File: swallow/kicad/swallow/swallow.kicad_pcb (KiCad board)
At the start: 2 copper layers, 35 parts, among them J1 Raspberry_Pi_2_3, J10 evens, J2 echo2, J3 ground, J4 VCC, J5 echo3, J6 echo4, J7 echo1, J8 power terminal, J9 odds, SW1 SW_Push

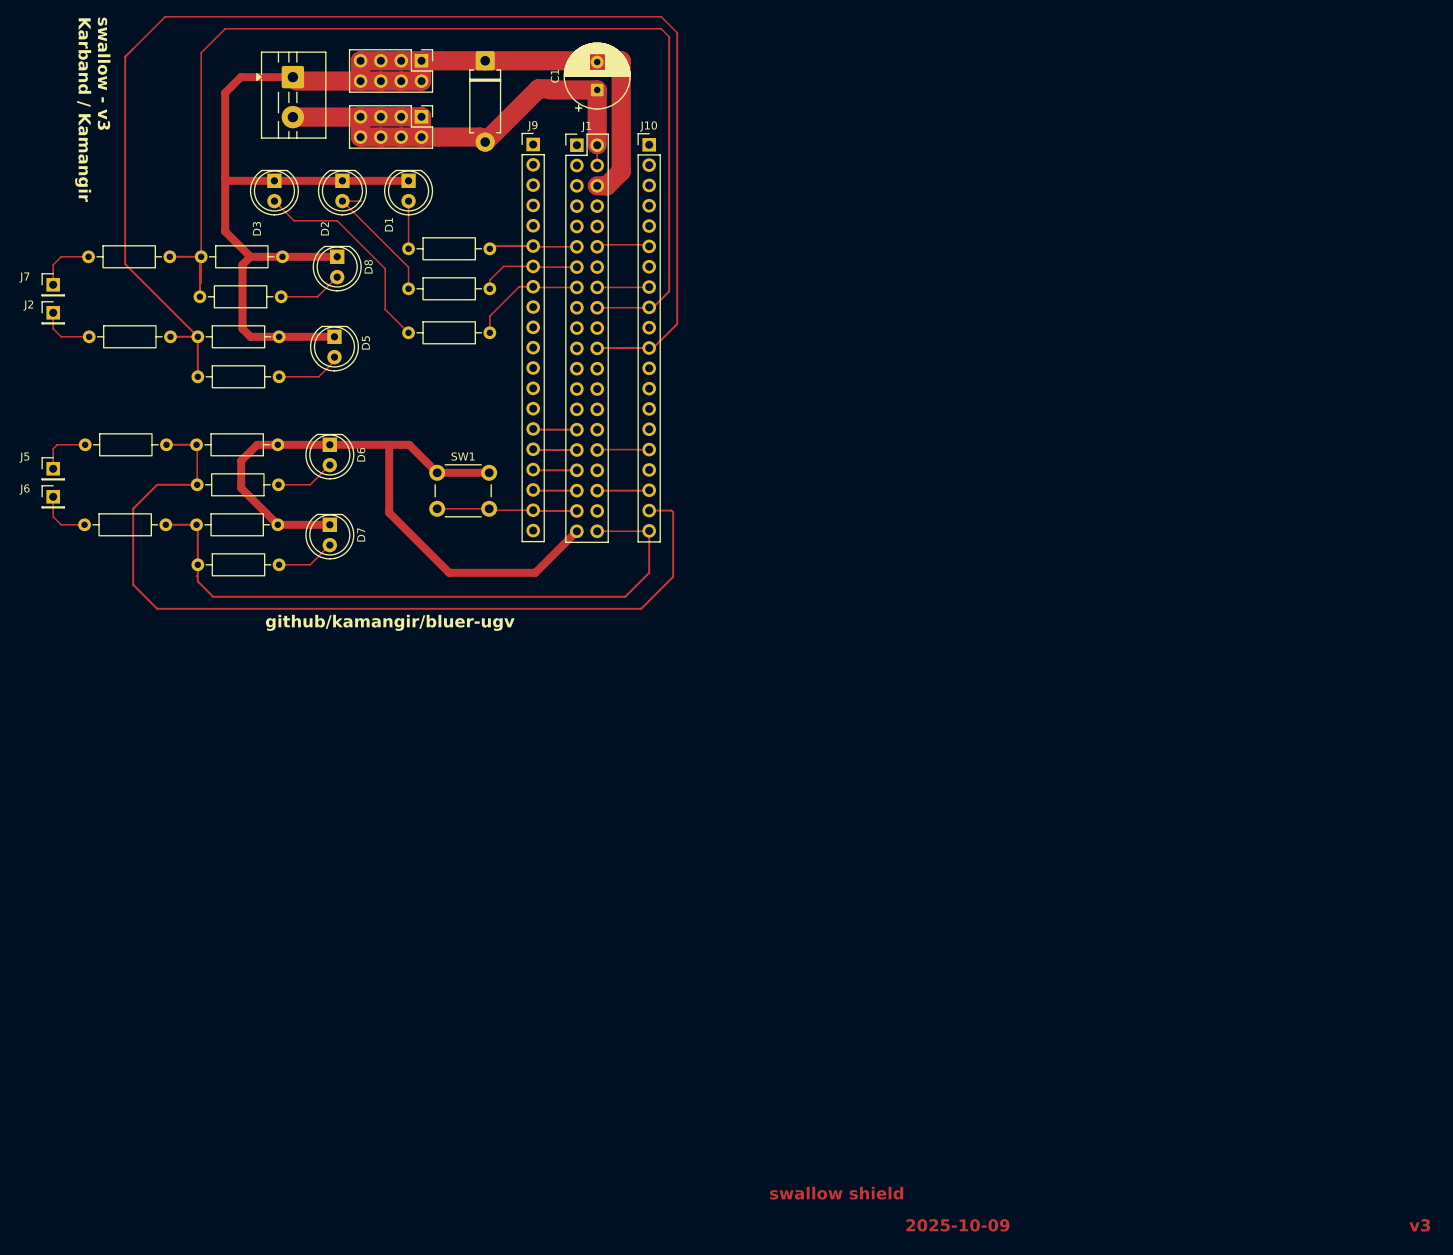
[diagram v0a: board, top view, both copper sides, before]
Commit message: ++ - kamangir/bolt#746
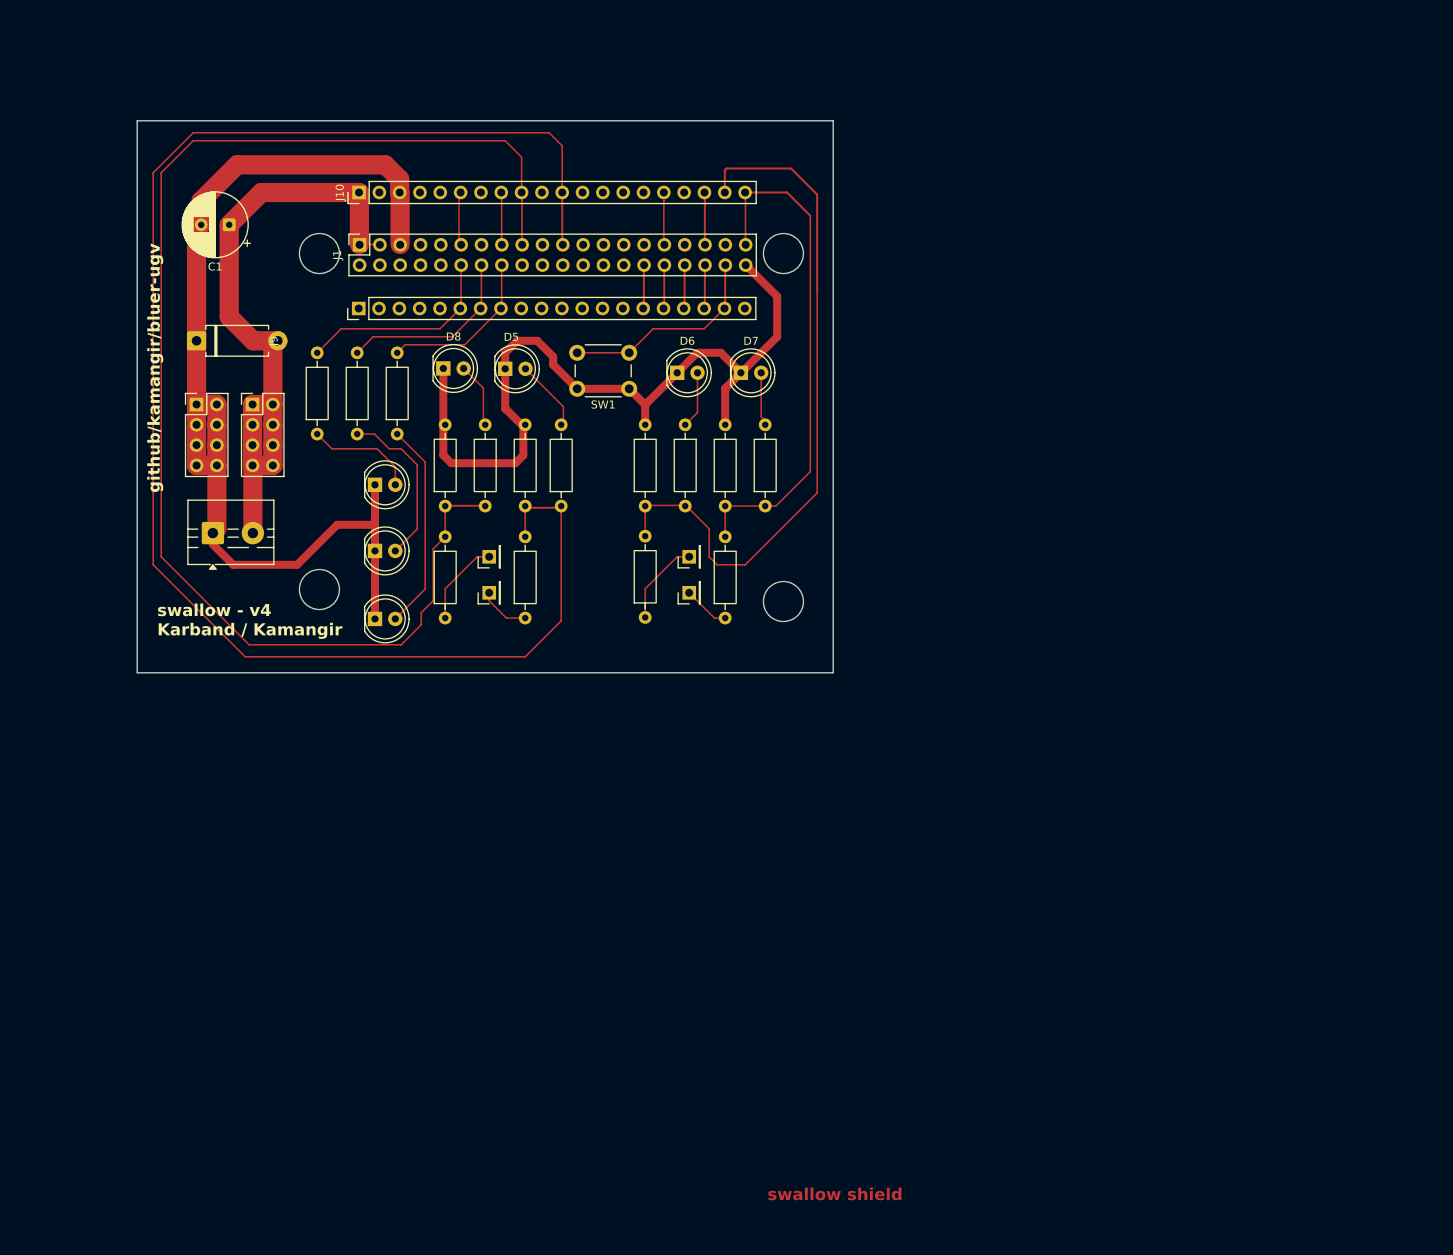
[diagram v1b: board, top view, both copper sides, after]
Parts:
- J1: footprint Connector_PinHeader_2.54mm:PinHeader_2x20_P2.54mm_Vertical -> Connector_PinSocket_2.54mm:PinSocket_2x20_P2.54mm_Vertical
- moved R12 80.9 mm to (183.5, 117.2), turned to 90 degrees
- moved J6 80.4 mm to (179.0, 114.0), turned to 90 degrees
- moved J5 80.3 mm to (179.0, 109.5), turned to 90 degrees
- moved R9 73.3 mm to (173.5, 117.1), turned to 90 degrees
- moved R11 71.3 mm to (188.5, 103.2), turned to 90 degrees
- moved R10 66.1 mm to (183.5, 103.2), turned to 90 degrees
- moved R4 64.9 mm to (158.5, 117.2), turned to 90 degrees
- moved J2 64.8 mm to (154.0, 114.0), turned to 90 degrees
- moved J7 64.2 mm to (154.0, 109.5), turned to 90 degrees
- moved R15 63.5 mm to (148.5, 117.2), turned to 90 degrees
- moved J8 57.9 mm to (119.5, 106.5), turned to 0 degrees
- moved R7 56.6 mm to (173.5, 103.2), turned to 90 degrees
- moved D3 56.2 mm to (139.7, 117.3), turned to 0 degrees
- moved D7 54.8 mm to (185.5, 86.5), turned to 0 degrees
- moved R8 51.4 mm to (178.5, 93.0), turned to -90 degrees
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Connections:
- J1 pad 11: Net-(D4-A) -> Net-(J1-GPIO17)
- J1 pad 13: Net-(D1-K) -> Net-(J1-GPIO27)
- J10 pad 1: unconnected-(J10-Pin_1-Pad1) -> Net-(D4-A)
- J10 pad 3: unconnected-(J10-Pin_3-Pad3) -> Net-(D1-K)
- J9 pad 6: Net-(D4-A) -> Net-(J1-GPIO17)
- J9 pad 7: Net-(D1-K) -> Net-(J1-GPIO27)
- R1 pad 2: Net-(D4-A) -> Net-(J1-GPIO17)
- R2 pad 2: Net-(D1-K) -> Net-(J1-GPIO27)
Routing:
- net Net-(J1-GPIO25): track 166.9 -> 196.6 mm
- net Net-(D1-K): track 257.7 -> 230.3 mm
- net Net-(J1-GPIO24): track 140.5 -> 167.1 mm
- net Net-(J1-GPIO17): track 0.00 -> 25.6 mm
- net Net-(J1-GPIO27): track 0.00 -> 23.1 mm
- net Net-(J1-GPIO20/MOSI1): track 109.1 -> 87.4 mm
- net Net-(J1-GPIO21/SCLK1): track 81.2 -> 64.3 mm
- net Net-(D4-A): track 67.3 -> 83.0 mm
- net Net-(J1-GPIO26): track 17.6 -> 26.8 mm
- net Net-(D1-A): track 5.96 -> 13.7 mm
- net Net-(J1-GPIO22): track 14.4 -> 20.6 mm
- net Net-(J1-PWM0/GPIO12): track 5.54 -> 0.00 mm
- net Net-(J1-GCLK2/GPIO6): track 5.50 -> 11.0 mm
- net Net-(D2-A): track 16.8 -> 21.0 mm
- net Net-(J5-Pin_1): track 6.71 -> 10.7 mm
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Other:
- board outline added: 87 x 69 mm
- board text added: "swallow - v4 Karband / Kamangir"
- board text removed: "2025-10-09"
- board text removed: "swallow - v3 Karband / Kamangir"
- board text removed: "v3"
